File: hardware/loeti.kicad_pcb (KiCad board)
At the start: 2 copper layers, 69.3 x 41.9 mm, 53 parts, among them J1 USB_C_Receptacle_USB2.0, J2 AudioJack3, J3 20021112-00014T1LF, Q1 BC817, Q2 BC817, Q3 BC807, Q4 Si4825DDY, DMG4435SSS, IRF939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, SW1 D6R, U1 AP2204R-3.3, U2 STUSB4500QTR, U3 STM32F030K6Tx, U4 TLV333-DBV, U5 INA239

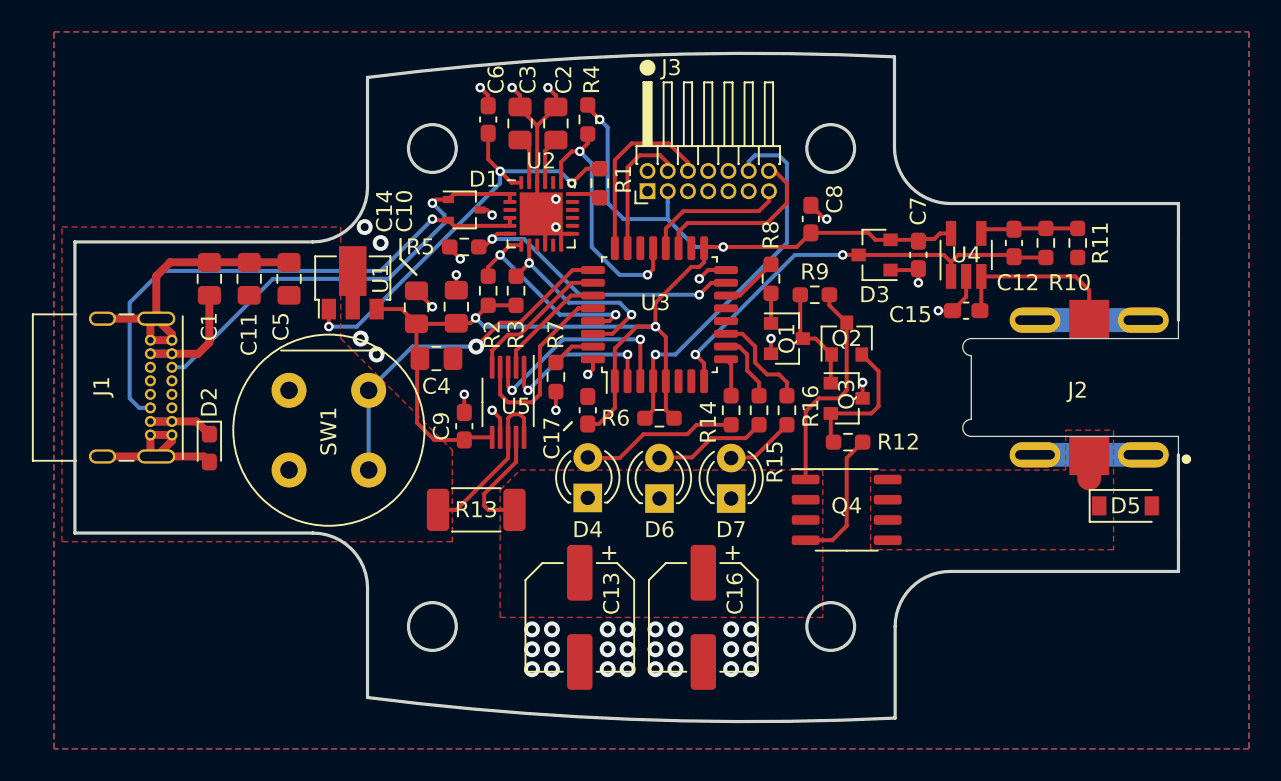
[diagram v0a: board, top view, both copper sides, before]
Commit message: production version, v5
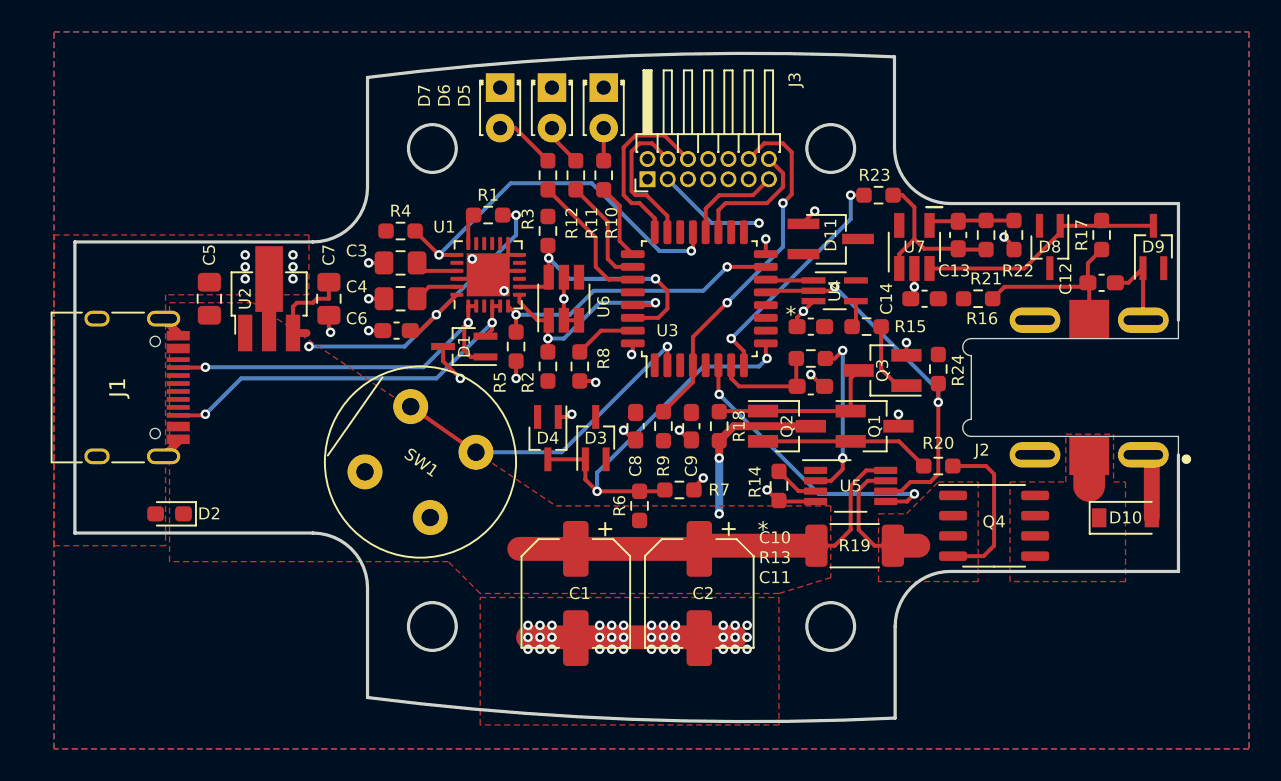
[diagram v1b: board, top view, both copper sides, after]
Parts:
- removed the C10 at (77.8, -33.8)
- removed the C14 at (75.2, -33.7)
- removed the C5 at (67.2, -35.5)
- removed the R12 at (102.3, -25.2)
- removed the R8 at (97.5, -35.5)
- added D11: BZX84Cxx, Package_TO_SOT_SMD:TSOT-23_HandSoldering, F.Cu at (101.2, -38.0)
- added D4: BAS16W, Package_TO_SOT_SMD:SOT-323_SC-70_Handsoldering, F.Cu at (83.5, -25.5)
- added D8: BAS16W, Package_TO_SOT_SMD:SOT-323_SC-70_Handsoldering, F.Cu at (115.0, -37.5)
- added D9: BAS16W, Package_TO_SOT_SMD:SOT-323_SC-70_Handsoldering, F.Cu at (121.5, -37.5)
- added R13: 1k, Resistor_SMD:R_0603_1608Metric_Pad0.98x0.95mm_HandSolder, F.Cu at (100.0, -30.5)
- added R14: 25k, Resistor_SMD:R_0603_1608Metric_Pad0.98x0.95mm_HandSolder, F.Cu at (98.0, -22.5)
- added R15: 1k, Resistor_SMD:R_0603_1608Metric_Pad0.98x0.95mm_HandSolder, F.Cu at (103.5, -32.5)
- added R16: 1M, Resistor_SMD:R_0603_1608Metric_Pad0.98x0.95mm_HandSolder, F.Cu at (110.5, -34.2)
- added R17: 10k, Resistor_SMD:R_0603_1608Metric_Pad0.98x0.95mm_HandSolder, F.Cu at (118.2, -38.2)
- added R20: 20, Resistor_SMD:R_0603_1608Metric_Pad0.98x0.95mm_HandSolder, F.Cu at (108.0, -23.8)
- added R23: 10k, Resistor_SMD:R_0603_1608Metric_Pad0.98x0.95mm_HandSolder, F.Cu at (104.2, -40.8)
- added R24: 10k, Resistor_SMD:R_0603_1608Metric_Pad0.98x0.95mm_HandSolder, F.Cu at (108.0, -29.8)
- added R6: 10k, Resistor_SMD:R_0603_1608Metric_Pad0.98x0.95mm_HandSolder, F.Cu at (89.2, -21.2)
- added R7: 1k, Resistor_SMD:R_0603_1608Metric_Pad0.98x0.95mm_HandSolder, F.Cu at (91.8, -22.2)
- added U4: 74AHC1G08, Package_TO_SOT_SMD:SOT-353_SC-70-5_Handsoldering, F.Cu at (101.5, -34.8)
- added U6: TMP100, Package_TO_SOT_SMD:SOT-23-6_Handsoldering, F.Cu at (84.5, -34.2)
- C10: renamed from C9; value 0.1μF -> 100n
- C11: value 1μF 25V -> 100n; footprint Capacitor_SMD:C_0805_2012Metric_Pad1.18x1.45mm_HandSolder -> Capacitor_SMD:C_0603_1608Metric_Pad1.08x0.95mm_HandSolder
- C12: renamed from C15; value 0.1μF -> 100n
- C13: renamed from C12; value 0.1μF -> 100n
- C14: renamed from C17; value 0.1μF -> 100n
- C3: renamed from C2; value 1μF 25V -> 1u
- C4: renamed from C3; value 1μF 25V -> 1u
- C5: renamed from C1; value 1μF 25V -> 4.7u
- C6: value 0.1μF -> 100n
- C7: renamed from C4; value 1μF 25V -> 4.7u
- C8: renamed from C7; value 0.1μF -> 100n
- C9: renamed from C8; value 0.1μF -> 100n
- D1: footprint Package_TO_SOT_SMD:SOT-323_SC-70 -> Package_TO_SOT_SMD:SOT-323_SC-70_Handsoldering
- D3: value BAT54S -> BAS16W; footprint Package_TO_SOT_SMD:SOT-23 -> Package_TO_SOT_SMD:SOT-323_SC-70_Handsoldering
- D5: renamed from D4; footprint LED_THT:LED_D3.0mm -> LED_THT:LED_D1.8mm_W3.3mm_H2.4mm
- D6, D7: footprint LED_THT:LED_D3.0mm -> LED_THT:LED_D1.8mm_W3.3mm_H2.4mm
- J1: value USB_C_Receptacle_USB2.0 -> GCT USB4105; footprint Connector_USB:USB_C_Receptacle_GCT_USB4085 -> Connector_USB:USB_C_Receptacle_HRO_TYPE-C-31-M-12
- Q1, Q2, Q3: footprint Package_TO_SOT_SMD:SOT-23 -> Package_TO_SOT_SMD:SOT-23_Handsoldering
- R10: renamed from R14; value 1k -> 10k
- R11: renamed from R15; value 1k -> 10k
- R12: renamed from R16; value 1k -> 10k
- R18: renamed from R9; value 1k -> 10k
- U2: renamed from U1; footprint Package_TO_SOT_SMD:SOT-89-3 -> Package_TO_SOT_SMD:SOT-89-3_Handsoldering
- U5: value INA239 -> INA301; footprint Package_SO:VSSOP-10_3x3mm_P0.5mm -> Package_SO:VSSOP-8_3.0x3.0mm_P0.65mm
- moved C11 35.9 mm to (100.0, -28.8), turned to 0 degrees
- moved D7 29.6 mm to (80.5, -47.5), turned to 270 degrees
- moved D6 26.7 mm to (83.8, -47.5), turned to 270 degrees
- moved D5 25.8 mm to (87.0, -47.5), turned to 270 degrees
- moved R19 23.9 mm to (102.8, -18.8)
- moved C10 22.6 mm to (100.0, -32.5), turned to 180 degrees
- moved C14 22.3 mm to (107.1, -34.2), turned to 180 degrees
- moved U5 22.1 mm to (102.5, -22.5), turned to 0 degrees
- moved R12 21.0 mm to (83.5, -42.0), turned to 270 degrees
- moved D3 20.9 mm to (86.5, -25.5), turned to 90 degrees
- moved C8 20.8 mm to (89.0, -26.2)
- moved R11 18.7 mm to (85.2, -42.0), turned to 270 degrees
- moved R10 16.8 mm to (87.0, -42.0), turned to 270 degrees
- moved C9 15.0 mm to (92.5, -26.2), turned to 270 degrees
- moved C6 14.4 mm to (74.0, -32.2), turned to 0 degrees
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- renumbered C13 to C1, C16 to C2, D5 to D10, R13 to R19, R10 to R21, R11 to R22, R7 to R8, R6 to R9, U2 to U1, U4 to U7
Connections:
- C1 pad 1: SHUNT- -> SHUNT+
- C11 pad 1: SHUNT+ -> ADC_IN1
- C13 pad 1: ADC_IN2 -> Net-(C13-Pad1)
- C2 pad 1: SHUNT- -> SHUNT+
- D3 pad 1: HEATER- -> ADC_IN3
- D3 pad 2: +3V3 -> (no net)
- D3 pad 3: ADC_IN2 -> +3V3
- Q2 pad 3: SHUNT- -> SHUNT+
- R18 pad 2: SHUNT- -> SHUNT+
- R21 pad 1: ADC_IN2 -> Net-(C13-Pad1)
- U3 pad 10: LED1 -> (no net)
- U3 pad 11: LED2 -> (no net)
- U3 pad 13: (no net) -> CURR_ALERT
- U3 pad 2: CURR_CS -> SW
- U3 pad 25: SW -> LED0
- U3 pad 26: SPI1_SCK -> LED1
- U3 pad 27: SPI1_MISO -> LED2
- U3 pad 28: SPI1_MOSI -> (no net)
- U3 pad 3: CURR_ALERT -> (no net)
- U3 pad 6: (no net) -> CURR_RESET
- U3 pad 7: (no net) -> ADC_IN1
- U3 pad 9: LED0 -> ADC_IN3
- U5 pad 1: CURR_CS -> +3V3
- U5 pad 2: SPI1_MISO -> Net-(R13-Pad2)
- U5 pad 3: CURR_ALERT -> Net-(R14-Pad2)
- U5 pad 4: SPI1_MOSI -> HEATER-
- U5 pad 5: SPI1_SCK -> CURR_RESET
- U5 pad 6: +3V3 -> CURR_ALERT
- U5 pad 7: HEATER- -> SHUNT-
- U7 pad 1: ADC_IN2 -> Net-(C13-Pad1)
- U7 pad 3: T+ -> Net-(D8-Pad1)
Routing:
- net +3V3: track 87.4 -> 12.9 mm, vias 4 -> 1
- net ADC_IN3: track 0.00 -> 24.7 mm, vias 0 -> 2
- net CURR_RESET: track 0.00 -> 18.7 mm, vias 0 -> 2
- net HEATER-: track 82.9 -> 65.7 mm, vias 47 -> 66
- net Net-(D8-Pad1): track 0.00 -> 15.7 mm
- net ADC_IN2: track 27.8 -> 15.0 mm
- net SHUNT-: track 21.0 -> 8.60 mm
- net SPI1_MOSI: track 11.9 -> 0.00 mm
- net Net-(C13-Pad1): track 0.00 -> 10.8 mm
- net Net-(R13-Pad2): track 0.00 -> 10.7 mm, vias 0 -> 2
- net CURR_CS: track 10.4 -> 0.00 mm, vias 2 -> 0
- net CURR_ALERT: track 13.6 -> 23.8 mm
- net CC2: track 34.3 -> 24.7 mm, vias 1 -> 2
- net SPI1_SCK: track 9.14 -> 0.00 mm
- net Net-(D5-Pad2): track 9.86 -> 2.05 mm
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- added copper zone on F.Cu, net +3V3
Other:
- net class Default: clearance 0.15 -> 0.127; trace_width 0.15 -> 0.25
- rule trace_clearance: 0.15 -> 0.127
- rule trace_min: 0.1 -> 0.127
- board text added: "*"
- board text added: "af 2021 v5"
- board text added: "löti"
- board text removed: "Löti mini"
- board text removed: "af 2021 v0.1"
